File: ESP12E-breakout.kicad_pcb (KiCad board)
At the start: 2 copper layers, 26.7 x 35.1 mm, 17 parts, among them P1 CONN_01X10, P3 CONN_01X08, SW1 RESET, SW2 FLASH, U1 ESP-12E, U2 AP1117

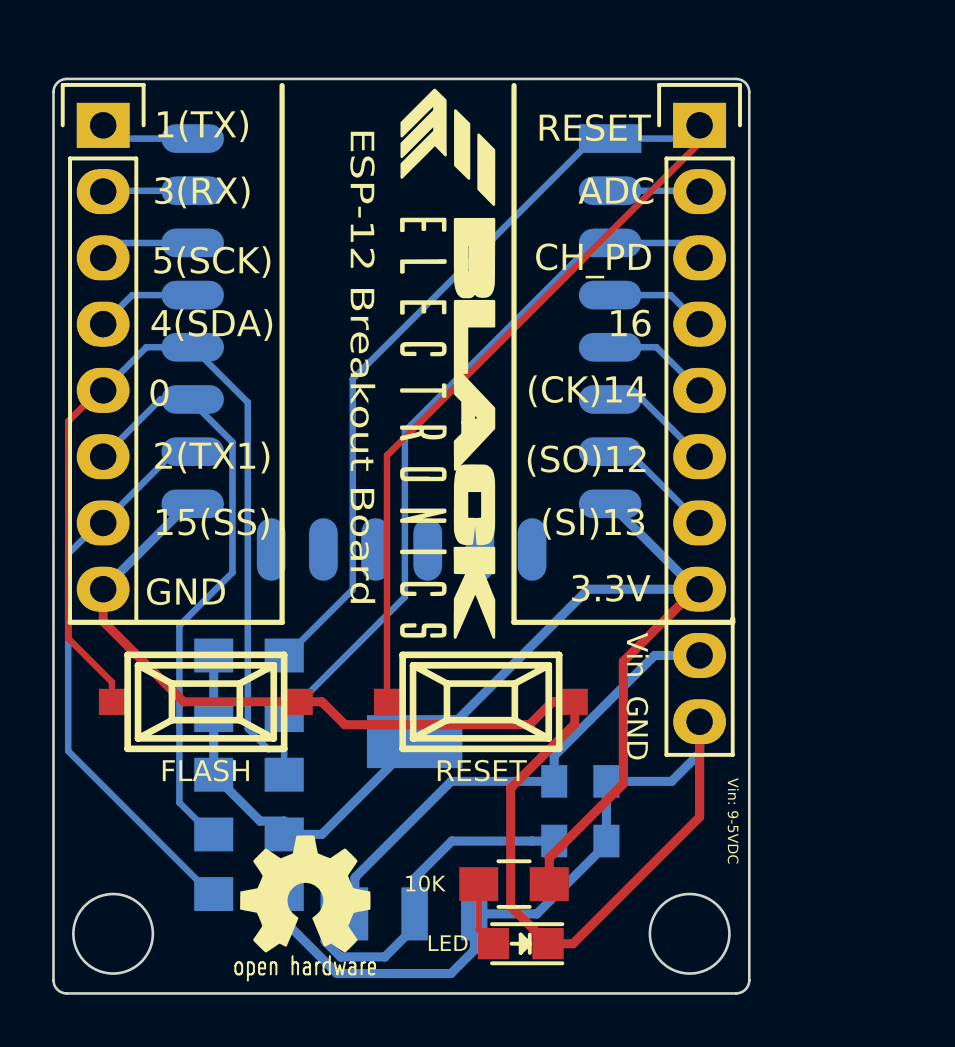
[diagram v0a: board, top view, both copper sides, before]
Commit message: Sent for Fab
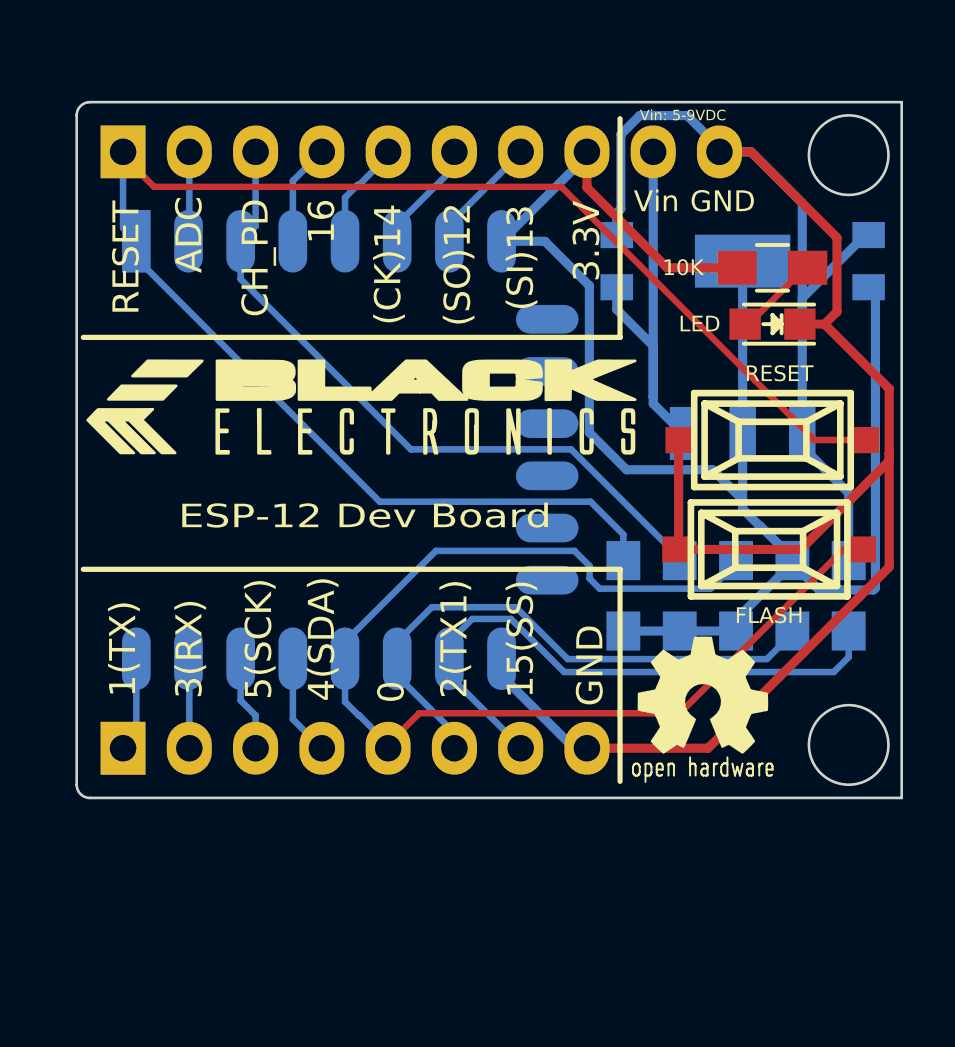
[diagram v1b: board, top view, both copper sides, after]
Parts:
- removed G0: LOGO, logo:3k5
- removed G1: LOGO, logo:oshw-logo-kicad-copper-10mm
- added P2: Logo, logo:3k5, F.Cu at (177.5, 56.5)
- added P4: OSHW logo, logo:oshw-logo-kicad-copper-10mm, F.Cu at (190.6, 67.6)
- P1, P3: moved to B.Cu
- U1: footprint ESP8266:ESP-12E -> ESP8266:ESP-12E_SilkOutline
- U2: value AP1117 -> 1117-3V3
- moved R5 25.7 mm to (196.2, 63.8), turned to 270 degrees
- moved D1 25.6 mm to (193.3, 53.3)
- moved R6 25.6 mm to (193.3, 51.2), turned to 180 degrees
- moved C2 24.8 mm to (197.0, 50.9), turned to 90 degrees
- moved P3 23.9 mm to (168.4, 69.6), turned to 270 degrees
- moved R4 22.7 mm to (194.1, 63.8), turned to 90 degrees
- moved SW2 22.4 mm to (193.2, 62.0), turned to 180 degrees
- moved U2 22.3 mm to (192.2, 54.2)
- moved P1 22.1 mm to (168.4, 46.7), turned to 270 degrees
- moved C1 20.0 mm to (187.3, 50.9), turned to 90 degrees
- moved R3 19.9 mm to (191.9, 63.8), turned to 270 degrees
- moved U1 18.6 mm to (168.9, 50.2), turned to 270 degrees
- moved R2 17.1 mm to (189.7, 63.8), turned to 270 degrees
- moved SW1 15.0 mm to (193.3, 57.8), turned to 0 degrees
- moved R1 14.5 mm to (187.6, 63.8), turned to 270 degrees
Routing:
- net GND: track 73.4 -> 86.2 mm
- net /0: track 35.6 -> 44.0 mm
- net /RESET: track 56.1 -> 61.5 mm
- net /5V: track 18.7 -> 16.1 mm
- net /15: track 21.8 -> 23.0 mm
- net /CH_PD: track 27.6 -> 26.5 mm
- net /2: track 23.1 -> 22.0 mm
- net /3V3: track 64.2 -> 65.3 mm
- net Net-(D1-Pad2): track 2.52 -> 3.29 mm
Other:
- board size 26.7 x 35.1 mm -> 31.6 x 26.7 mm
- board text added: "1117-3.3V"
- board text added: "Designed & Made in INDIA"
- board text added: "ESP-12 Dev Board"
- board text added: "Vin: 5-9VDC"
- board text removed: "ESP-12 Breakout Board"
- board text removed: "These pretzels are making me thirsty"
- board text removed: "Vin: 9-5VDC"
